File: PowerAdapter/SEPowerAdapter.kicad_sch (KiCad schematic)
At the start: 46 parts, among them J1 XOR, J2 ATX, J3 SE, J4 Classic, J5 VGA, U1 LM7905_TO220, U2 74LVC86AD, U3 74LVC86AD, U4 74HCT74D

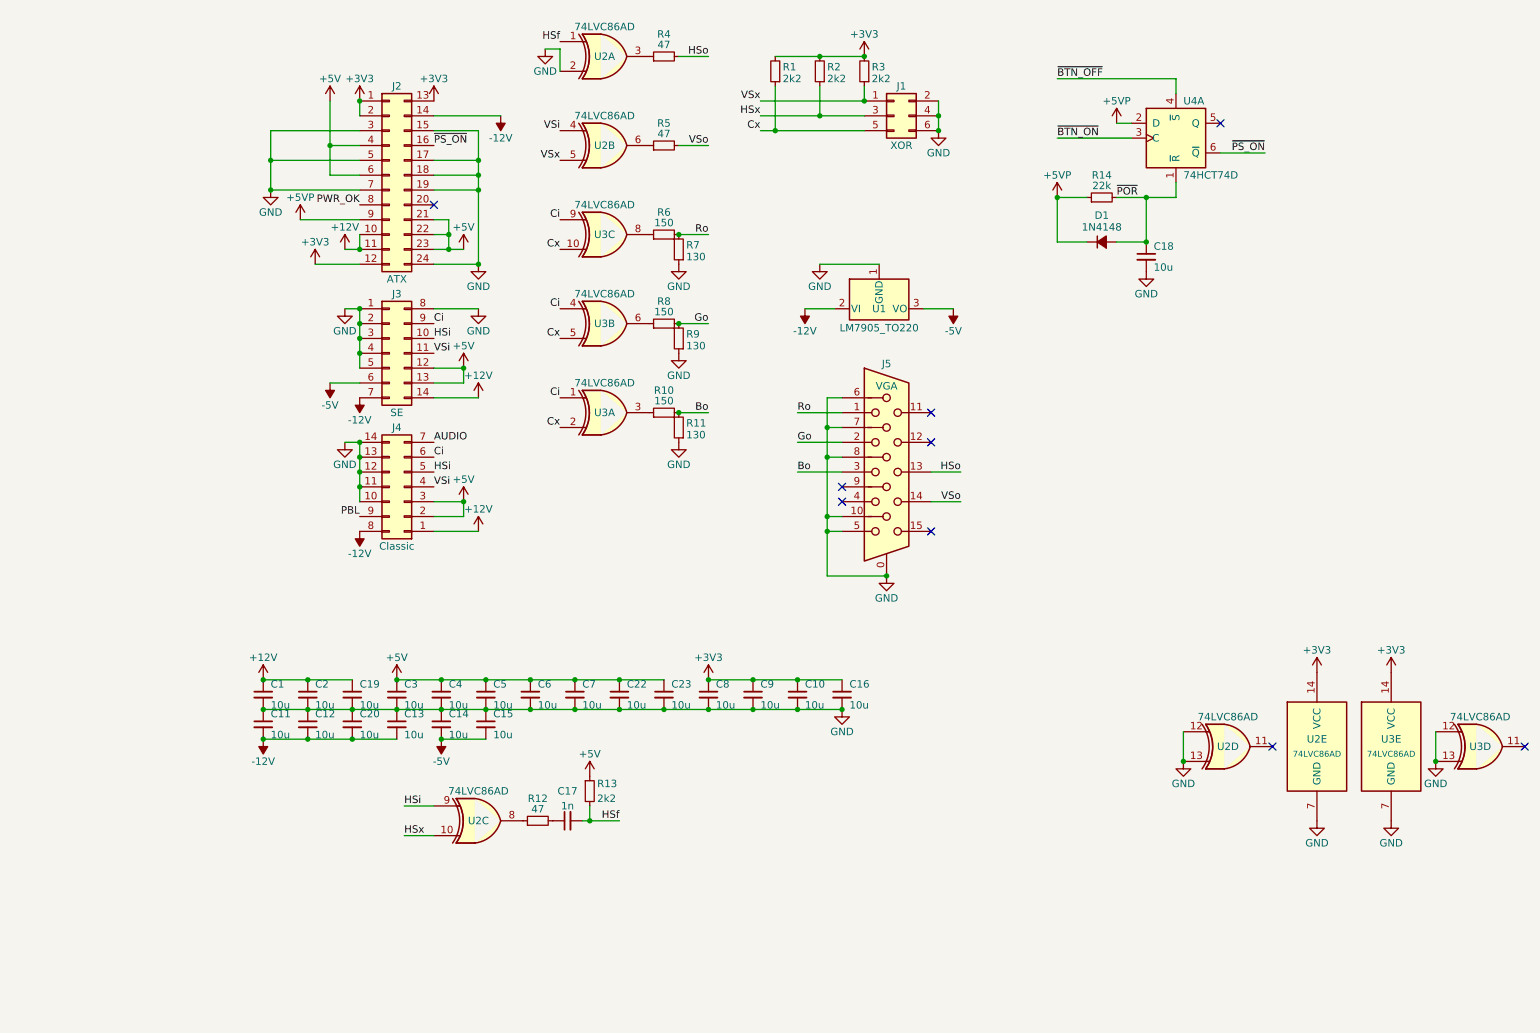
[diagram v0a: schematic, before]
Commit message: Toward final "A"
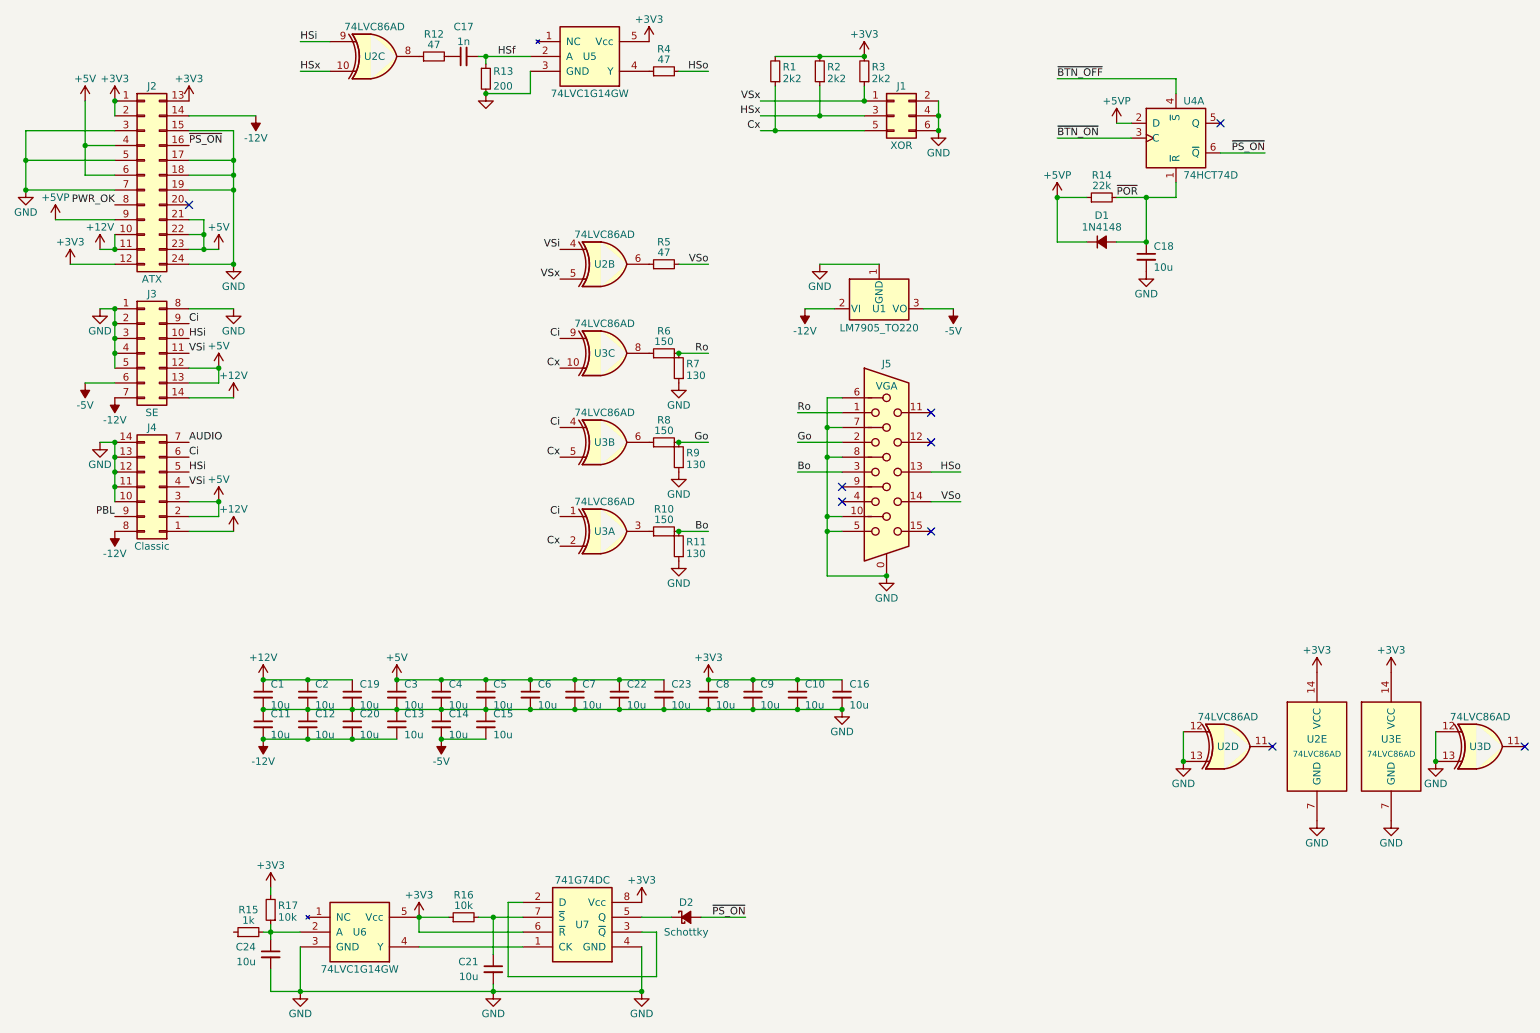
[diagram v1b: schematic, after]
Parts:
- removed unit 1 of U2
- added C21, C24: 10u, stdpads:C_0805, symbol Device:C_Small
- added D2: Schottky, stdpads:D_SOD-123, symbol Device:D_Schottky_Small_Filled
- added R15: 1k, stdpads:R_0805, symbol Device:R_Small
- added R16, R17: 10k, stdpads:R_0805, symbol Device:R_Small
- added U5, U6: 74LVC1G14GW, stdpads:SOT-353, symbol GW_Logic:741G04GW
- added U7: 741G74DC, stdpads:NXP_VSSOP-8_2.3x2mm, symbol GW_Logic:741G74DC
- R13: value 2k2 -> 200
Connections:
- net +3V3: now also R16.1, R17.2, U5.5 (Vcc), U6.5 (Vcc), U7.6 (~{R}), U7.8 (Vcc)
- net +5V: no longer R13.1
- net GND: now also R13.2, C21.2, C24.2, U5.3 (GND), U6.3 (GND), U7.4 (GND)
- net HSf: now also R13.1, U5.2 (A); no longer R13.2
- net ~{PS_ON}: now also D2.2 (A)
- net at R4.1: now also U5.4 (Y)
- new net: C24.1, R15.2, R17.1, U6.2 (A)
- new net: U6.4 (Y), U7.1 (CK)
- new net: U7.2 (D), U7.3 (~{Q})
- new net: D2.1 (K), U7.5 (Q)
- new net: C21.1, R16.2, U7.7 (~{S})
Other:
- moved on the sheet: C17, J2, J3, J4, R10, R11, R12, R13, R4, R5, R6, R7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
